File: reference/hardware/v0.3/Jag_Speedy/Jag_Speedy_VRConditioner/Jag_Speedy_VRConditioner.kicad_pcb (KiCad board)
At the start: 2 copper layers, 15 parts, among them IC1 MAX9926UAEE+, J1 Conn_02x04_Counter_Clockwise

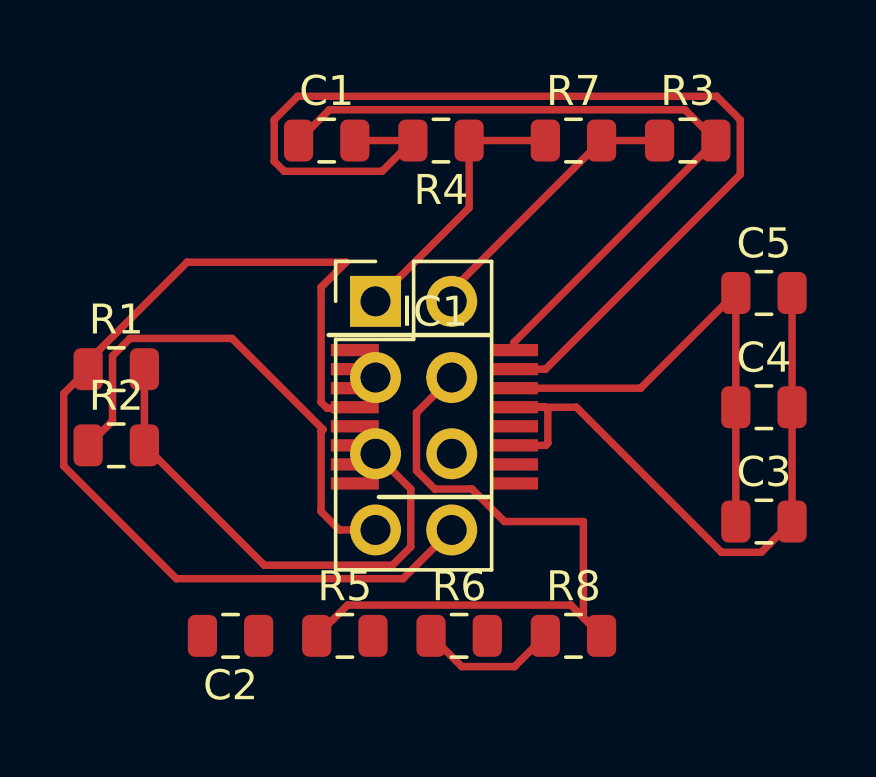
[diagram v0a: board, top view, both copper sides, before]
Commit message: VR PCB
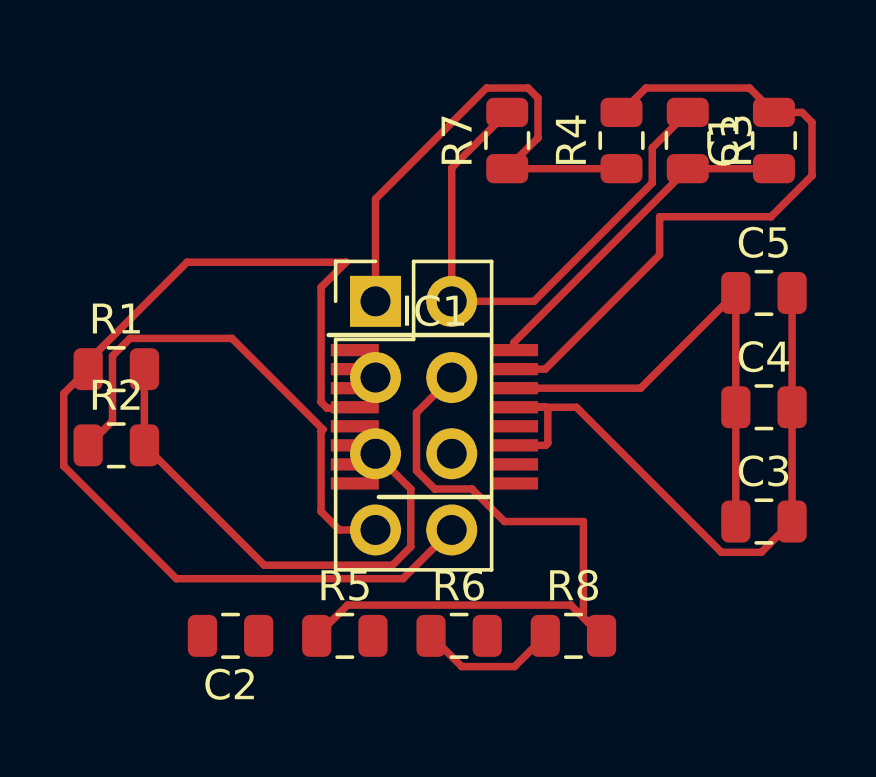
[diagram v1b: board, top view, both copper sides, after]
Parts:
- moved C1 14.9 mm to (149.9, 83.8), turned to 90 degrees
- moved R4 6.02 mm to (144.8, 83.8), turned to 90 degrees
- moved R7 2.21 mm to (141.0, 83.8), turned to 90 degrees
- turned R3 to 270 degrees
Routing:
- net Net-(C1-Pad2): track 36.7 -> 22.3 mm
- net Net-(C1-Pad1): track 24.5 -> 11.3 mm
- net VR1+: track 9.36 -> 18.2 mm
- net VR1-: track 9.19 -> 17.1 mm
